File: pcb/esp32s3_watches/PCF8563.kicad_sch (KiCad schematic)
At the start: 1 part, among them U6 PCF8563TS

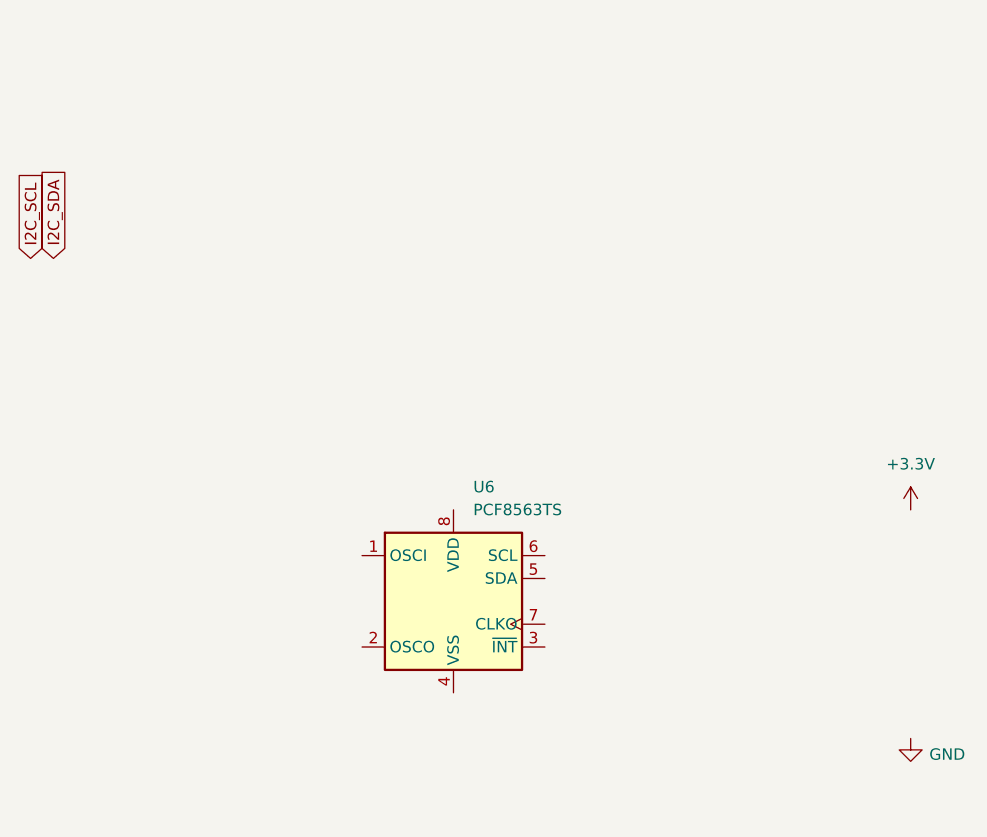
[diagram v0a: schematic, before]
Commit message: BOM file updates. Scheme complete.
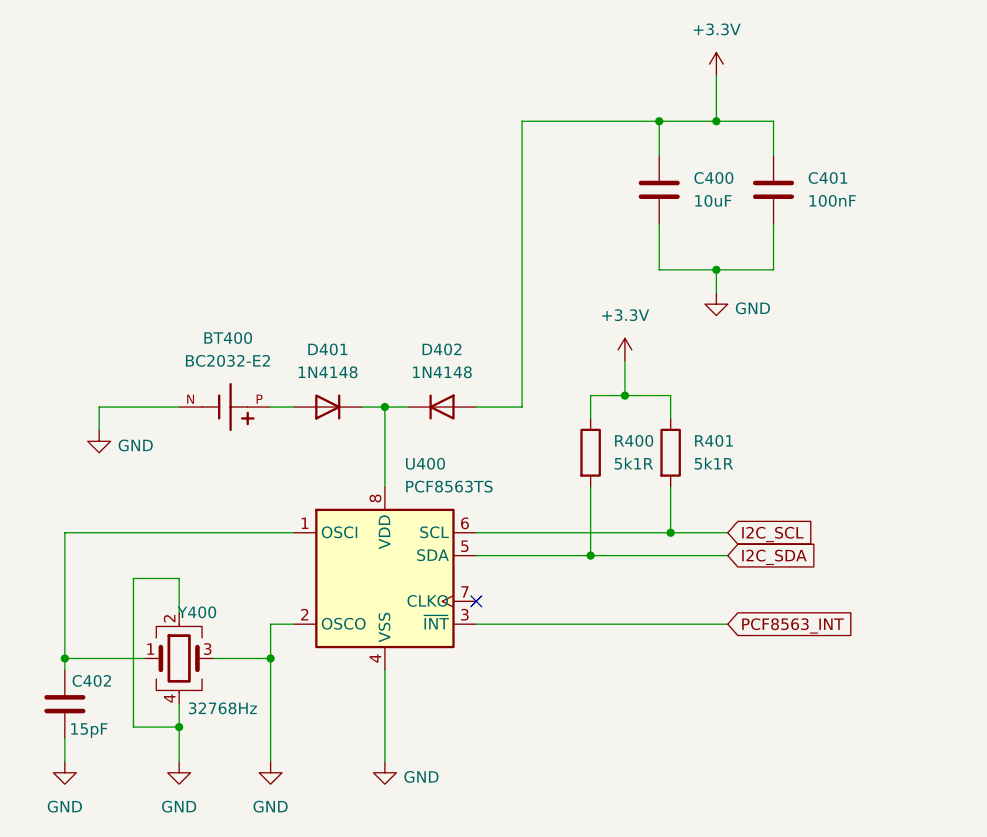
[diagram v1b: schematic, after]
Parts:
- added BT400: BC2032-E2, esp32s3_watches:MPD_BC2032-E2, symbol esp32s3_watches:BC2032-E2
- added C400: 10uF, Capacitor_SMD:C_0805_2012Metric, symbol Device:C
- added C401: 100nF, Capacitor_SMD:C_0603_1608Metric, symbol Device:C
- added C402: 15pF, Capacitor_SMD:C_0603_1608Metric, symbol Device:C
- added D401, D402: 1N4148, Diode_SMD:D_SOD-123, symbol Device:D
- added R400, R401: 5k1R, Resistor_SMD:R_0805_2012Metric, symbol Device:R
- added Y400: 32768Hz, Crystal:Crystal_SMD_3225-4Pin_3.2x2.5mm, symbol Device:Crystal_GND24
- U400: renamed from U6; Manufacturer (none) -> NXP Semicon; Manufacturer Product Number (none) -> PCF8563TS/5,118
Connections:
- net +3.3V: now also C400.1, C401.1, D402.2 (A), R400.1, R401.1
- net GND: now also U400.2 (OSCO), U400.4 (VSS), BT400.N, C400.2, C401.2, C402.2, Y400.2, Y400.3, Y400.4
- net I2C_SCL: now also U400.6 (SCL), R401.2
- net I2C_SDA: now also U400.5 (SDA), R400.2
- net at U400.1 (OSCI): now also C402.1, Y400.1
- net PCF8563_INT: now reaches U400.3 (~{INT})
- net at U400.8 (VDD): now also D401.1 (K), D402.1 (K)
- new net: BT400.P, D401.2 (A)
- no-connect marks 0 -> 1
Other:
- moved on the sheet: U400
